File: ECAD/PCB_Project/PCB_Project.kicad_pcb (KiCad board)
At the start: 2 copper layers, 105.4 x 113 mm, 2 parts

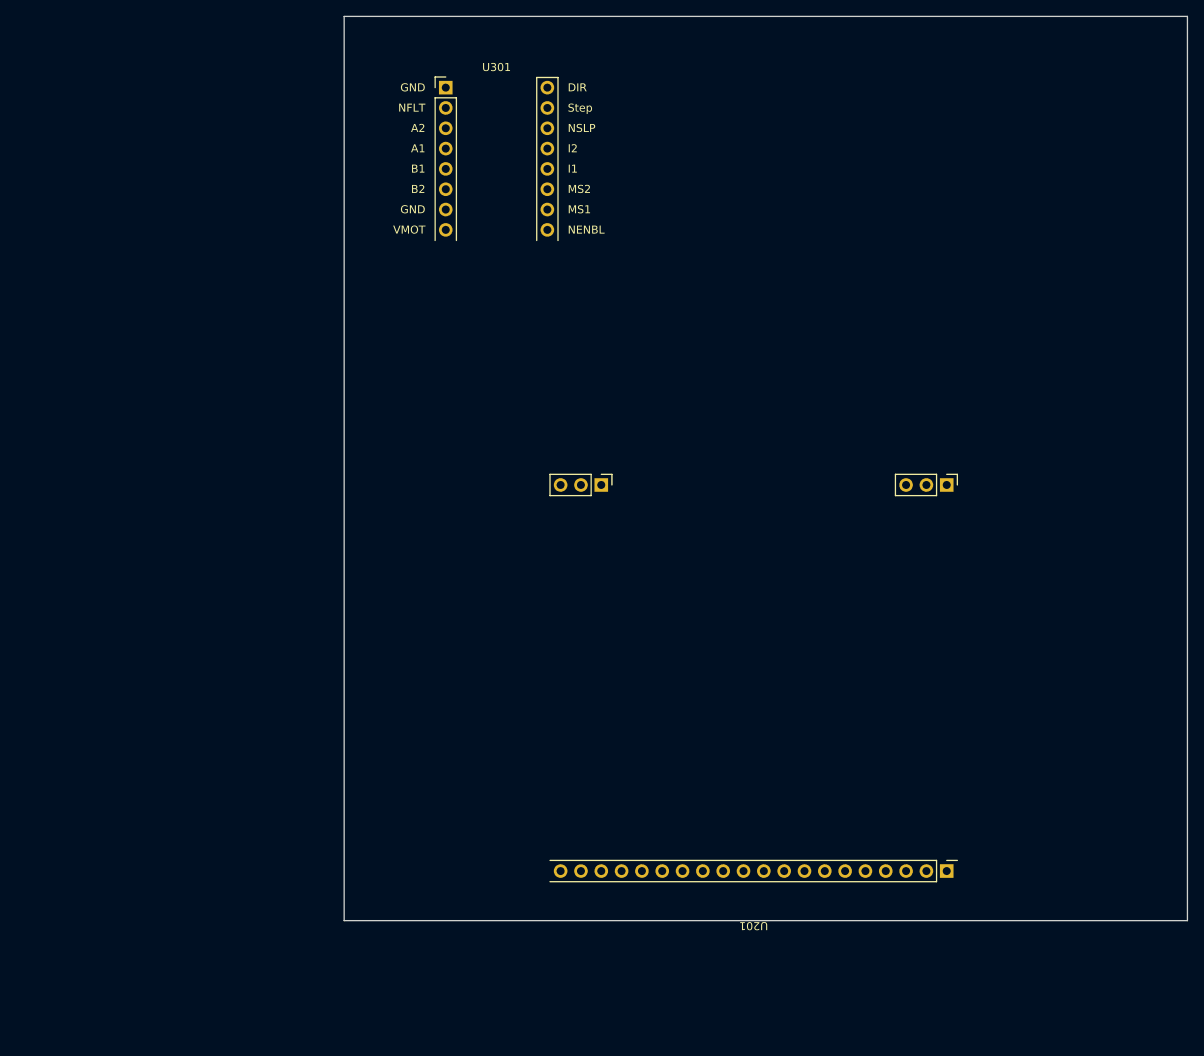
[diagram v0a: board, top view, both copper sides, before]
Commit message: First PCB Draft
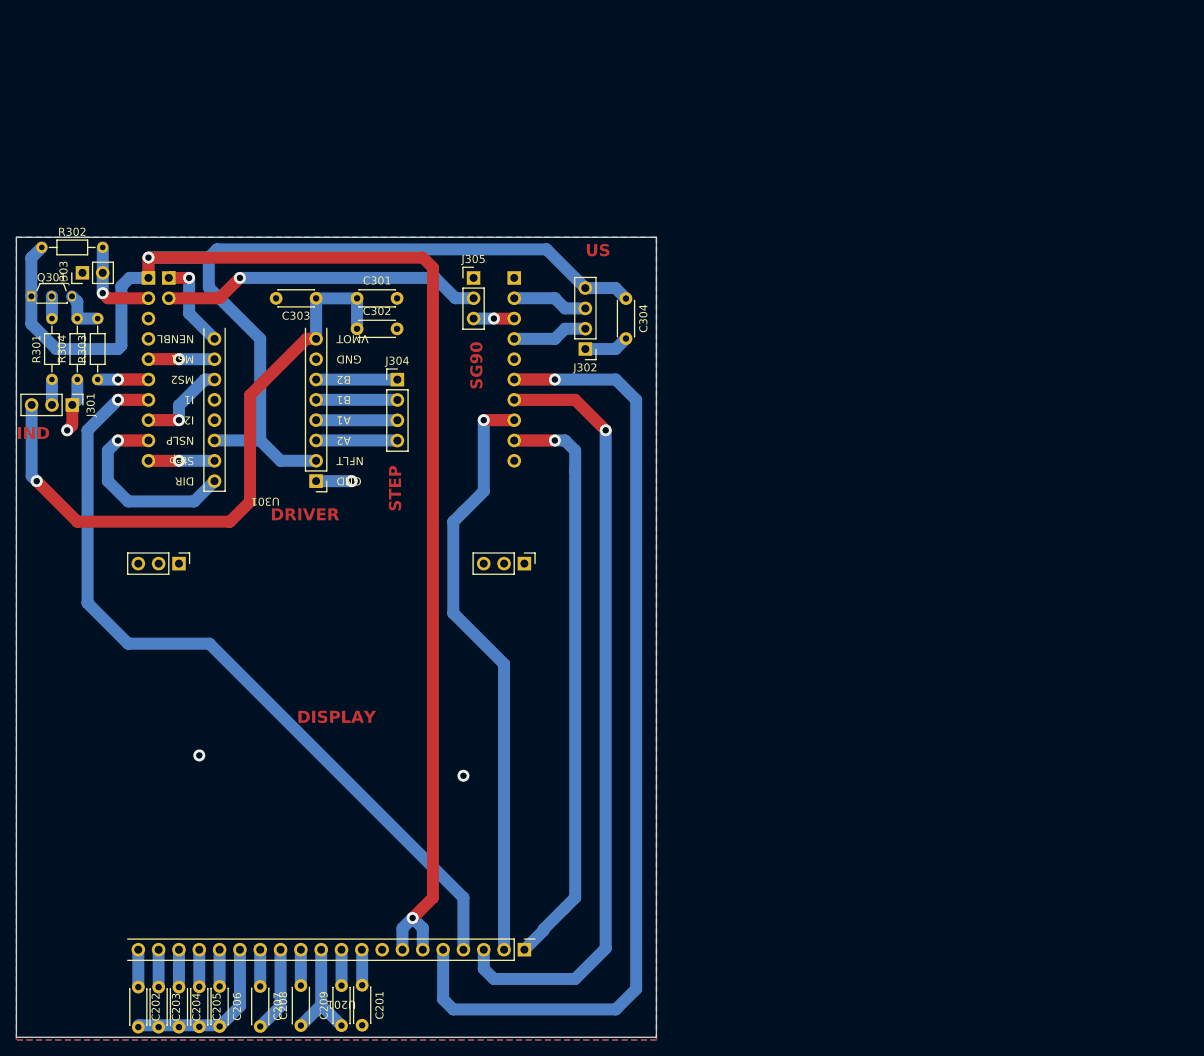
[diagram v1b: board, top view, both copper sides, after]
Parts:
- added C201: 1uF, Capacitor_THT:C_Disc_D4.3mm_W1.9mm_P5.00mm, F.Cu at (129.2, 159.2)
- added C202: 1uF, Capacitor_THT:C_Disc_D4.3mm_W1.9mm_P5.00mm, F.Cu at (101.3, 159.4)
- added C203: 1uF, Capacitor_THT:C_Disc_D4.3mm_W1.9mm_P5.00mm, F.Cu at (103.8, 159.4)
- added C204: 1uF, Capacitor_THT:C_Disc_D4.3mm_W1.9mm_P5.00mm, F.Cu at (106.3, 159.4)
- added C205: 1uF, Capacitor_THT:C_Disc_D4.3mm_W1.9mm_P5.00mm, F.Cu at (108.9, 159.4)
- added C206: 1uF, Capacitor_THT:C_Disc_D4.3mm_W1.9mm_P5.00mm, F.Cu at (111.4, 159.4)
- added C207: 1uF, Capacitor_THT:C_Disc_D4.3mm_W1.9mm_P5.00mm, F.Cu at (116.5, 159.4)
- added C208: 1uF, Capacitor_THT:C_Disc_D4.3mm_W1.9mm_P5.00mm, F.Cu at (121.6, 164.2)
- added C209: 1uF, Capacitor_THT:C_Disc_D4.3mm_W1.9mm_P5.00mm, F.Cu at (126.7, 164.2)
- added C301: 1uF, Capacitor_THT:C_Disc_D4.3mm_W1.9mm_P5.00mm, F.Cu at (128.6, 73.3)
- added C302: 100uF, Capacitor_THT:C_Disc_D4.3mm_W1.9mm_P5.00mm, F.Cu at (128.6, 77.2)
- added C303: 100nF, Capacitor_THT:C_Disc_D4.3mm_W1.9mm_P5.00mm, F.Cu at (123.5, 73.3)
- added C304: 100nF, Capacitor_THT:C_Disc_D4.3mm_W1.9mm_P5.00mm, F.Cu at (162.2, 73.4)
- added J301: Conn_01x03, Connector_PinHeader_2.54mm:PinHeader_1x03_P2.54mm_Vertical, F.Cu at (93.0, 86.7)
- added J302: Conn_01x04, Connector_PinHeader_2.54mm:PinHeader_1x04_P2.54mm_Vertical, F.Cu at (157.2, 79.7)
- added J303: Conn_01x02, Connector_PinHeader_2.54mm:PinHeader_1x02_P2.54mm_Vertical, F.Cu at (94.3, 70.2)
- added J304: Conn_01x04, Connector_PinHeader_2.54mm:PinHeader_1x04_P2.54mm_Vertical, F.Cu at (133.7, 83.5)
- added J305: Conn_01x03, Connector_PinHeader_2.54mm:PinHeader_1x03_P2.54mm_Vertical, F.Cu at (143.2, 70.8)
- added J401: Conn_01x10, Connector_PinSocket_2.54mm:PinSocket_1x10_P2.54mm_Vertical, B.Cu at (102.5, 70.8)
- added J402: Conn_01x10, Connector_PinSocket_2.54mm:PinSocket_1x10_P2.54mm_Vertical, B.Cu at (148.3, 70.8)
- added J403: Conn_01x02, Connector_PinHeader_2.54mm:PinHeader_1x02_P2.54mm_Vertical, B.Cu at (105.1, 70.8)
- added Q301: NPN, Package_TO_SOT_THT:TO-92S_Wide, F.Cu at (87.9, 73.1)
- added R301: 100k, Resistor_THT:R_Axial_DIN0204_L3.6mm_D1.6mm_P7.62mm_Horizontal, F.Cu at (90.5, 83.5)
- added R302: R, Resistor_THT:R_Axial_DIN0204_L3.6mm_D1.6mm_P7.62mm_Horizontal, F.Cu at (89.2, 67.0)
- added R303: 10k, Resistor_THT:R_Axial_DIN0204_L3.6mm_D1.6mm_P7.62mm_Horizontal, F.Cu at (96.2, 83.5)
- added R304: 10k, Resistor_THT:R_Axial_DIN0204_L3.6mm_D1.6mm_P7.62mm_Horizontal, F.Cu at (93.7, 83.5)
- moved U201 53.7 mm to (125.4, 161.1)
- moved U301 53.5 mm to (124.8, 97.5), turned to 180 degrees
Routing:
- net +3V3: track 0.00 -> 266.0 mm, vias 0 -> 2
- net /Display/DISPLAY.SDI: track 0.00 -> 121.9 mm, vias 0 -> 1
- net /Display/DISPLAY.SCL: track 0.00 -> 99.5 mm, vias 0 -> 1
- net /Display/DISPLAY.A0: track 0.00 -> 97.5 mm, vias 0 -> 1
- net +12V: track 0.00 -> 78.1 mm, vias 0 -> 1
- net /Display/DISPLAY.NRST: track 0.00 -> 74.2 mm, vias 0 -> 1
- net /Display/DISPLAY.NCS: track 0.00 -> 73.2 mm, vias 0 -> 1
- net GND: track 0.00 -> 49.3 mm, vias 0 -> 5
- net +5V: track 0.00 -> 40.2 mm, vias 0 -> 1
- net /MCU/Driver.DIR: track 0.00 -> 24.9 mm, vias 0 -> 1
- net Net-(U201-CAP1N): track 0.00 -> 14.1 mm
- net /MCU/LDR_Analog: track 0.00 -> 11.7 mm, vias 0 -> 1
- net /MCU/Driver.MS2: track 0.00 -> 11.4 mm, vias 0 -> 1
- net Net-(U201-CAP2P): track 0.00 -> 10.6 mm
- net Net-(J304-Pin_3): track 0.00 -> 10.2 mm
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- added copper zone on B.Cu, net GND
- added copper zone on F.Cu, net GND
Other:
- board size 105.4 x 113 mm -> 80 x 100 mm
- board text added: "DISPLAY"
- board text added: "DRIVER"
- board text added: "IND"
- board text added: "SG90"
- board text added: "STEP"
- board text added: "US"
